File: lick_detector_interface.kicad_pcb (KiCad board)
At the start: 2 copper layers, 7 x 14.5 mm, 7 parts, among them P1 CONN_FFC_8_RA, U1 ADXL313

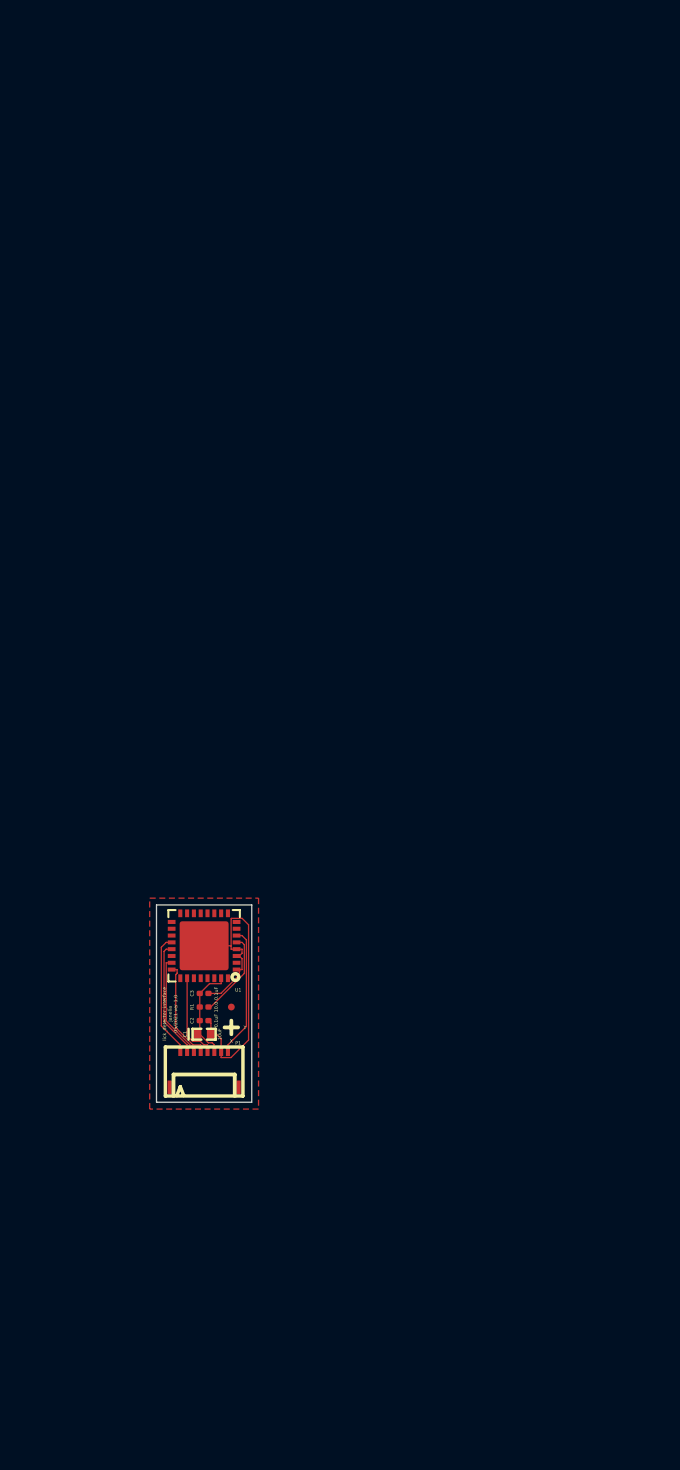
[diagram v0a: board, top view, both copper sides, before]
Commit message: Finished v1.0
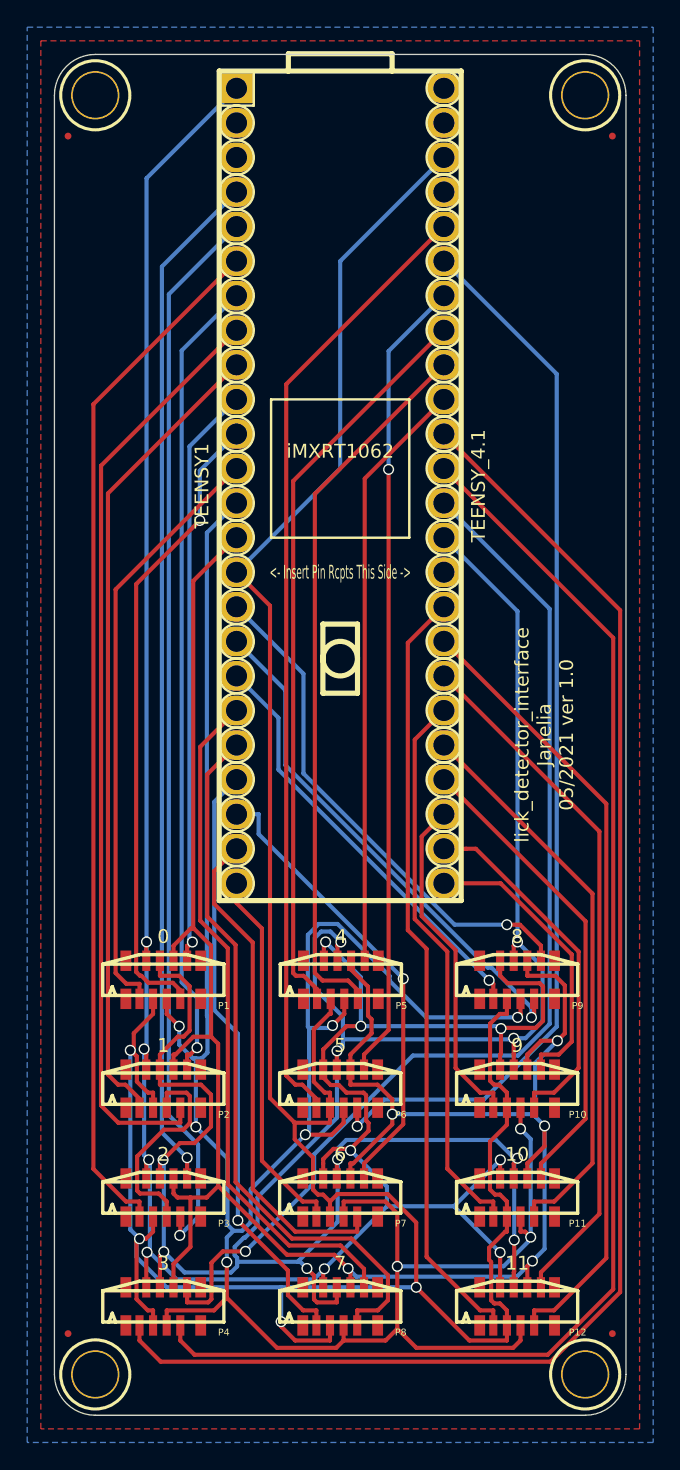
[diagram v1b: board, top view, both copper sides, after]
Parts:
- removed C1: 10uF, lick_detector_interface:SM0402_POL
- removed C2, C3: 0.1uF, lick_detector_interface:SM0201
- removed R1: 10.0, lick_detector_interface:SM0201
- removed U1: ADXL313, lick_detector_interface:LFCSP-32-1EP_5x5mm_P0.5mm_EP3.6x3.6mm
- added FID2: FIDUCIAL, lick_detector_interface:FIDUCIAL, F.Cu at (180.0, 35.0)
- added FID3: FIDUCIAL, lick_detector_interface:FIDUCIAL, F.Cu at (180.0, 123.0)
- added FID4: FIDUCIAL, lick_detector_interface:FIDUCIAL, F.Cu at (140.0, 123.0)
- added MH1: MOUNTING_HOLE_4-40, lick_detector_interface:MOUNTING_HOLE_4-40, F.Cu at (142.0, 32.0)
- added MH2: MOUNTING_HOLE_4-40, lick_detector_interface:MOUNTING_HOLE_4-40, F.Cu at (178.0, 32.0)
- added MH3: MOUNTING_HOLE_4-40, lick_detector_interface:MOUNTING_HOLE_4-40, F.Cu at (178.0, 126.0)
- added MH4: MOUNTING_HOLE_4-40, lick_detector_interface:MOUNTING_HOLE_4-40, F.Cu at (142.0, 126.0)
- added P10: CONN_FFC_8_VERT, lick_detector_interface:Molex_FFC_1x8_P0.5mm_Vertical, F.Cu at (173.0, 105.0)
- added P11: CONN_FFC_8_VERT, lick_detector_interface:Molex_FFC_1x8_P0.5mm_Vertical, F.Cu at (173.0, 113.0)
- added P12: CONN_FFC_8_VERT, lick_detector_interface:Molex_FFC_1x8_P0.5mm_Vertical, F.Cu at (173.0, 121.0)
- added P2: CONN_FFC_8_VERT, lick_detector_interface:Molex_FFC_1x8_P0.5mm_Vertical, F.Cu at (147.0, 105.0)
- added P3: CONN_FFC_8_VERT, lick_detector_interface:Molex_FFC_1x8_P0.5mm_Vertical, F.Cu at (147.0, 113.0)
- added P4: CONN_FFC_8_VERT, lick_detector_interface:Molex_FFC_1x8_P0.5mm_Vertical, F.Cu at (147.0, 121.0)
- added P5: CONN_FFC_8_VERT, lick_detector_interface:Molex_FFC_1x8_P0.5mm_Vertical, F.Cu at (160.1, 97.0)
- added P6: CONN_FFC_8_VERT, lick_detector_interface:Molex_FFC_1x8_P0.5mm_Vertical, F.Cu at (160.0, 105.0)
- added P7: CONN_FFC_8_VERT, lick_detector_interface:Molex_FFC_1x8_P0.5mm_Vertical, F.Cu at (160.0, 113.0)
- added P8: CONN_FFC_8_VERT, lick_detector_interface:Molex_FFC_1x8_P0.5mm_Vertical, F.Cu at (160.0, 121.0)
- added P9: CONN_FFC_8_VERT, lick_detector_interface:Molex_FFC_1x8_P0.5mm_Vertical, F.Cu at (173.0, 97.0)
- added TEENSY1: TEENSY_4.1, lick_detector_interface:TEENSY_4.1, F.Cu at (160.0, 48.0)
- P1: value CONN_FFC_8_RA -> CONN_FFC_8_VERT; footprint lick_detector_interface:Molex_FFC_1x8_P0.5mm_RA -> lick_detector_interface:Molex_FFC_1x8_P0.5mm_Vertical
- moved FID1 65.1 mm to (140.0, 35.0)
- moved P1 6.05 mm to (147.0, 97.0)
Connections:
- P1 pad 1: /INT1 -> /~CS_0
- P1 pad 2: /INT2 -> /GND
- P1 pad 3: /MISO -> /VAA
- P1 pad 4: /MOSI -> /SCK
- P1 pad 5: /SCK -> /MOSI
- P1 pad 6: VAA -> /MISO
- P1 pad 7: GND -> /INT2_0
- P1 pad 8: /~CS -> /INT1_0
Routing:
- net /VAA: track 0.00 -> 214.2 mm, vias 0 -> 4
- net /MOSI: track 7.53 -> 205.4 mm, vias 0 -> 9
- net /GND: track 0.00 -> 191.5 mm, vias 0 -> 11
- net /SCK: track 6.47 -> 178.1 mm, vias 0 -> 10
- net /MISO: track 7.74 -> 164.8 mm, vias 0 -> 5
- net /~CS_3: track 0.00 -> 107.6 mm
- net /INT2_3: track 0.00 -> 100.8 mm
- net /INT1_3: track 0.00 -> 80.5 mm, vias 0 -> 1
- net /INT2_2: track 0.00 -> 79.0 mm, vias 0 -> 1
- net /INT2_5: track 0.00 -> 78.7 mm, vias 0 -> 1
- net /~CS_2: track 0.00 -> 76.5 mm
- net /INT1_2: track 0.00 -> 75.5 mm, vias 0 -> 1
- net /~CS_5: track 0.00 -> 70.8 mm
- net /INT2_1: track 0.00 -> 68.5 mm
- net /~CS_1: track 0.00 -> 59.8 mm
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- added copper zone on B.Cu, net /GND
- added copper zone on F.Cu, net /VAA
- removed copper zone on F.Cu, net GND
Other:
- board size 7 x 14.5 mm -> 42 x 100 mm
- net class POWER: clearance 0.0762 -> 0.2032; trace_width 0.0762 -> 0.3048; via_dia 0.254 -> 0.8128; via_drill 0.1524 -> 0.6096
- net class SIGNAL: clearance 0.0762 -> 0.2032; trace_width 0.0762 -> 0.3048; via_dia 0.254 -> 0.8128; via_drill 0.1524 -> 0.6096
- board text removed: "X"
- board text removed: "Y"
